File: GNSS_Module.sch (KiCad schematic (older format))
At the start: 8 parts, among them J14 GPS Shield, J15 GPS_Transmission_Conn, U11 ublox_SAM-M8Q

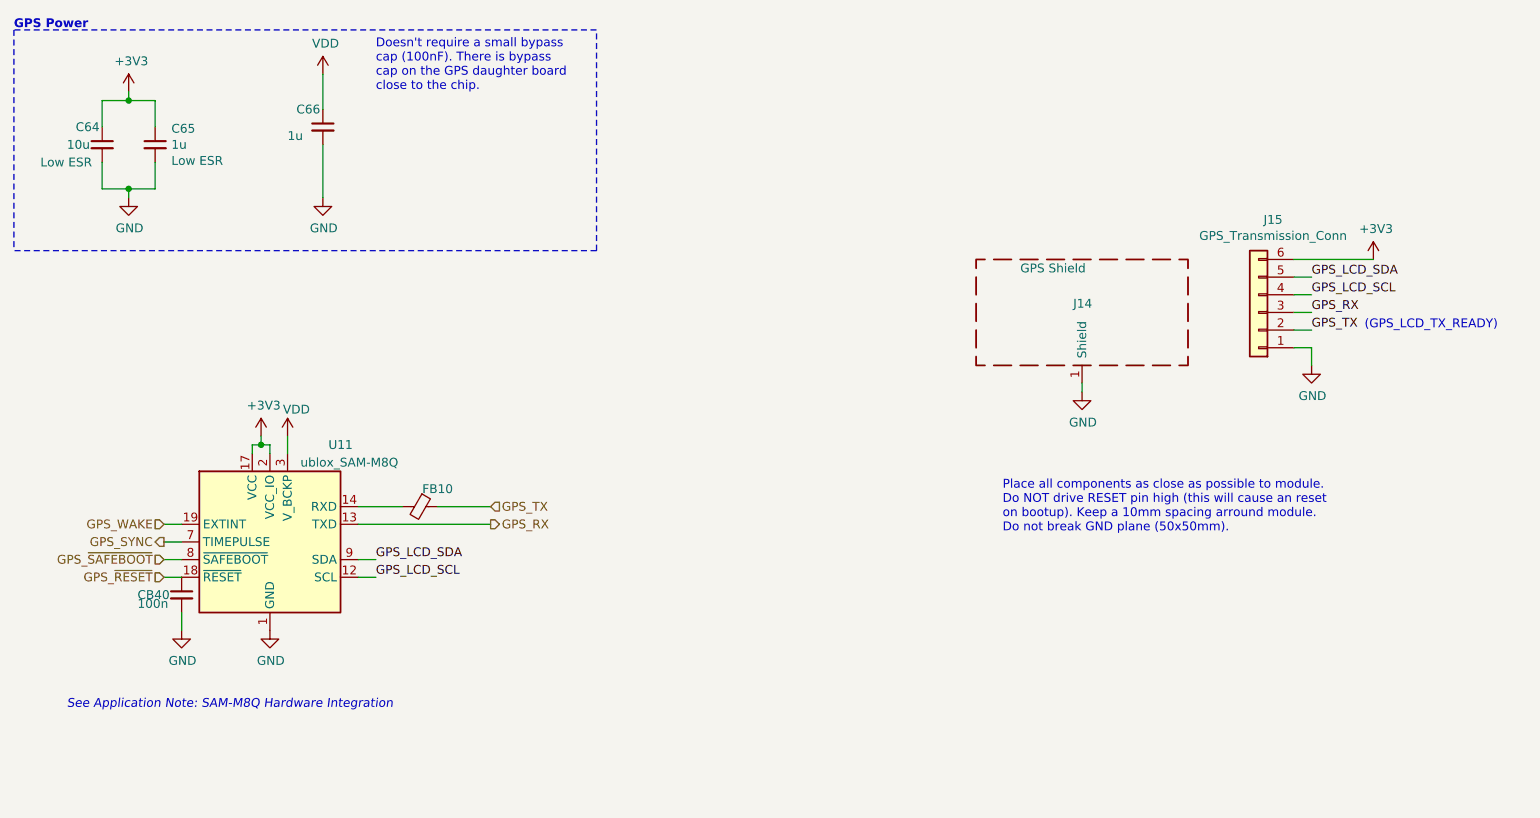
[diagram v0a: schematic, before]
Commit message: Major Commit with Final PCB Design
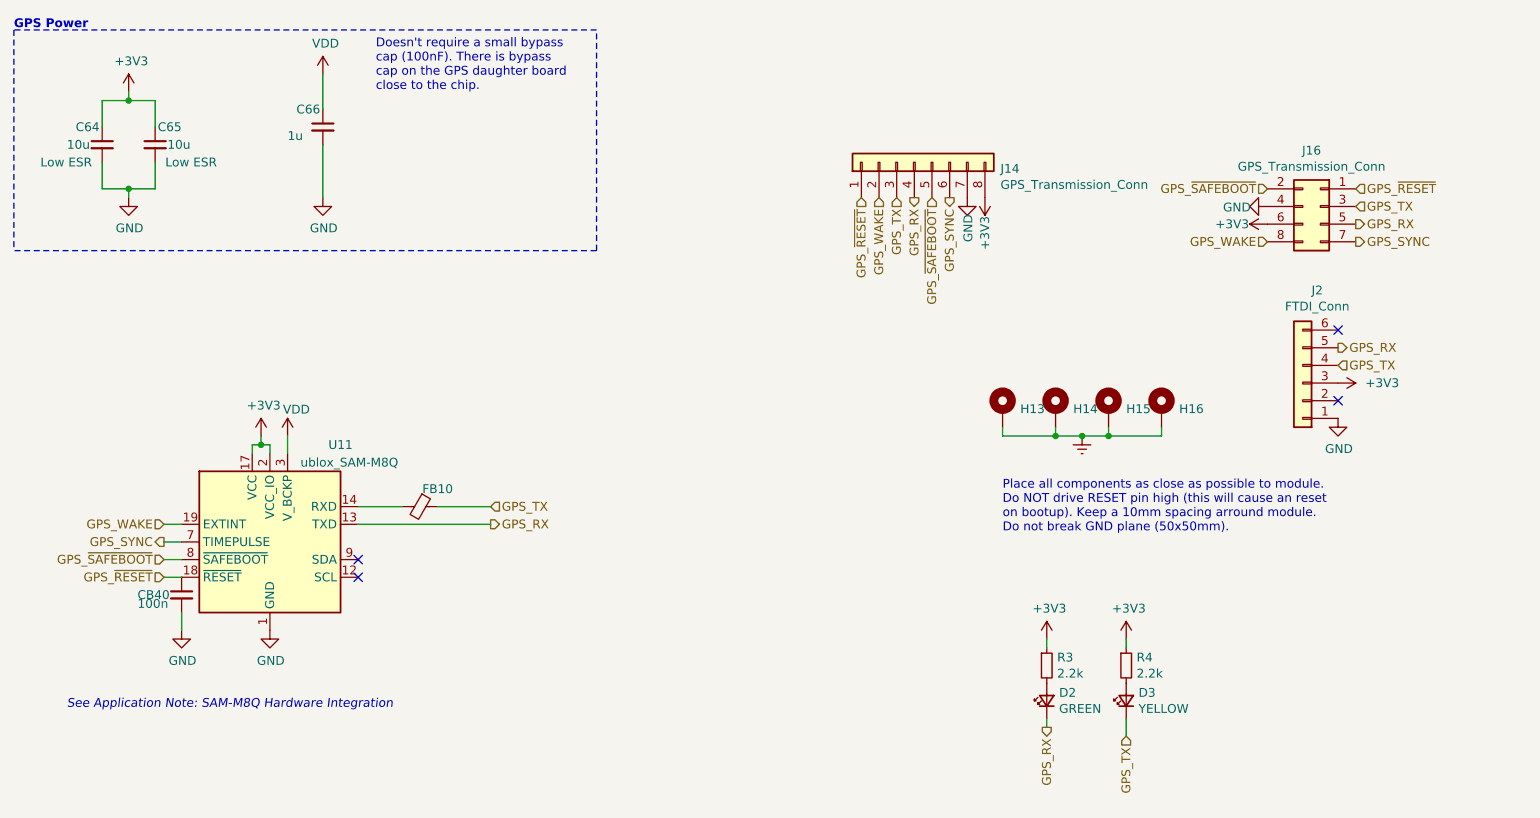
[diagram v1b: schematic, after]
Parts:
- removed J14: GPS Shield, RF_Shielding:Wuerth_36103505_50x50mm, symbol Device:RF_Shield_One_Piece
- removed J15: GPS_Transmission_Conn, Connector_PinHeader_2.54mm:PinHeader_1x06_P2.54mm_Vertical, symbol Connector_Generic:Conn_01x06
- added D2: GREEN, LED_SMD:LED_0603_1608Metric_Pad1.05x0.95mm_HandSolder, symbol Device:LED_Small
- added D3: YELLOW, LED_SMD:LED_0603_1608Metric_Pad1.05x0.95mm_HandSolder, symbol Device:LED_Small
- added H13, H14, H15, H16: MountingHole_Pad, MountingHole:MountingHole_4.3mm_M4_Pad_Via, symbol Mechanical:MountingHole_Pad
- added J14: GPS_Transmission_Conn, Connector_PinHeader_1.27mm:PinHeader_1x08_P1.27mm_Vertical, symbol Connector_Generic:Conn_01x08
- added J16: GPS_Transmission_Conn, Connector_PinHeader_1.27mm:PinHeader_2x04_P1.27mm_Vertical, symbol Connector_Generic:Conn_02x04_Odd_Even
- added J2: FTDI_Conn, Connector_PinHeader_2.54mm:PinHeader_1x06_P2.54mm_Vertical, symbol Connector_Generic:Conn_01x06
- added R3, R4: 2.2k, Resistor_SMD:R_0603_1608Metric_Pad1.05x0.95mm_HandSolder, symbol Device:R_Small
- C65: value 1u -> 10u; footprint Capacitor_SMD:C_0603_1608Metric_Pad1.05x0.95mm_HandSolder -> Capacitor_SMD:C_0805_2012Metric_Pad1.15x1.40mm_HandSolder; MPN C0603C105K8RACTU -> C0805C106K9PACTU
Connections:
- net +3V3: now also J14.8 (Pin_8), J16.6 (Pin_6), J2.3 (Pin_3), R3.1, R4.1
- net GND: now also J14.7 (Pin_7), J16.4 (Pin_4), J2.1 (Pin_1)
- net GPS_RX: now also D2.1 (K), J14.4 (Pin_4), J16.5 (Pin_5), J2.5 (Pin_5)
- net GPS_SYNC: now also J14.6 (Pin_6), J16.7 (Pin_7)
- net GPS_TX: now also D3.1 (K), J14.3 (Pin_3), J16.3 (Pin_3), J2.4 (Pin_4)
- net GPS_WAKE: now also J14.2 (Pin_2), J16.8 (Pin_8)
- net GPS_~RESET: now also J14.1 (Pin_1), J16.1 (Pin_1)
- net GPS_~SAFEBOOT: now also J14.5 (Pin_5), J16.2 (Pin_2)
- net GPS_LCD_SCL: no longer names the net of U11.12 (SCL)
- net GPS_LCD_SDA: no longer names the net of U11.9 (SDA)
- new net: D2.2 (A), R3.2
- new net: D3.2 (A), R4.2
- new net Earth: H13.1, H14.1, H15.1, H16.1
- no-connect marks 0 -> 4
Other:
- note removed: "(GPS_LCD_TX_READY)"
